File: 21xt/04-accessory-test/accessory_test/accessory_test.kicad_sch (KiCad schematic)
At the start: 10 parts, among them J1 Conn_01x44, J2 Conn_01x01, J3 Conn_01x02, U3 Teensy4.1

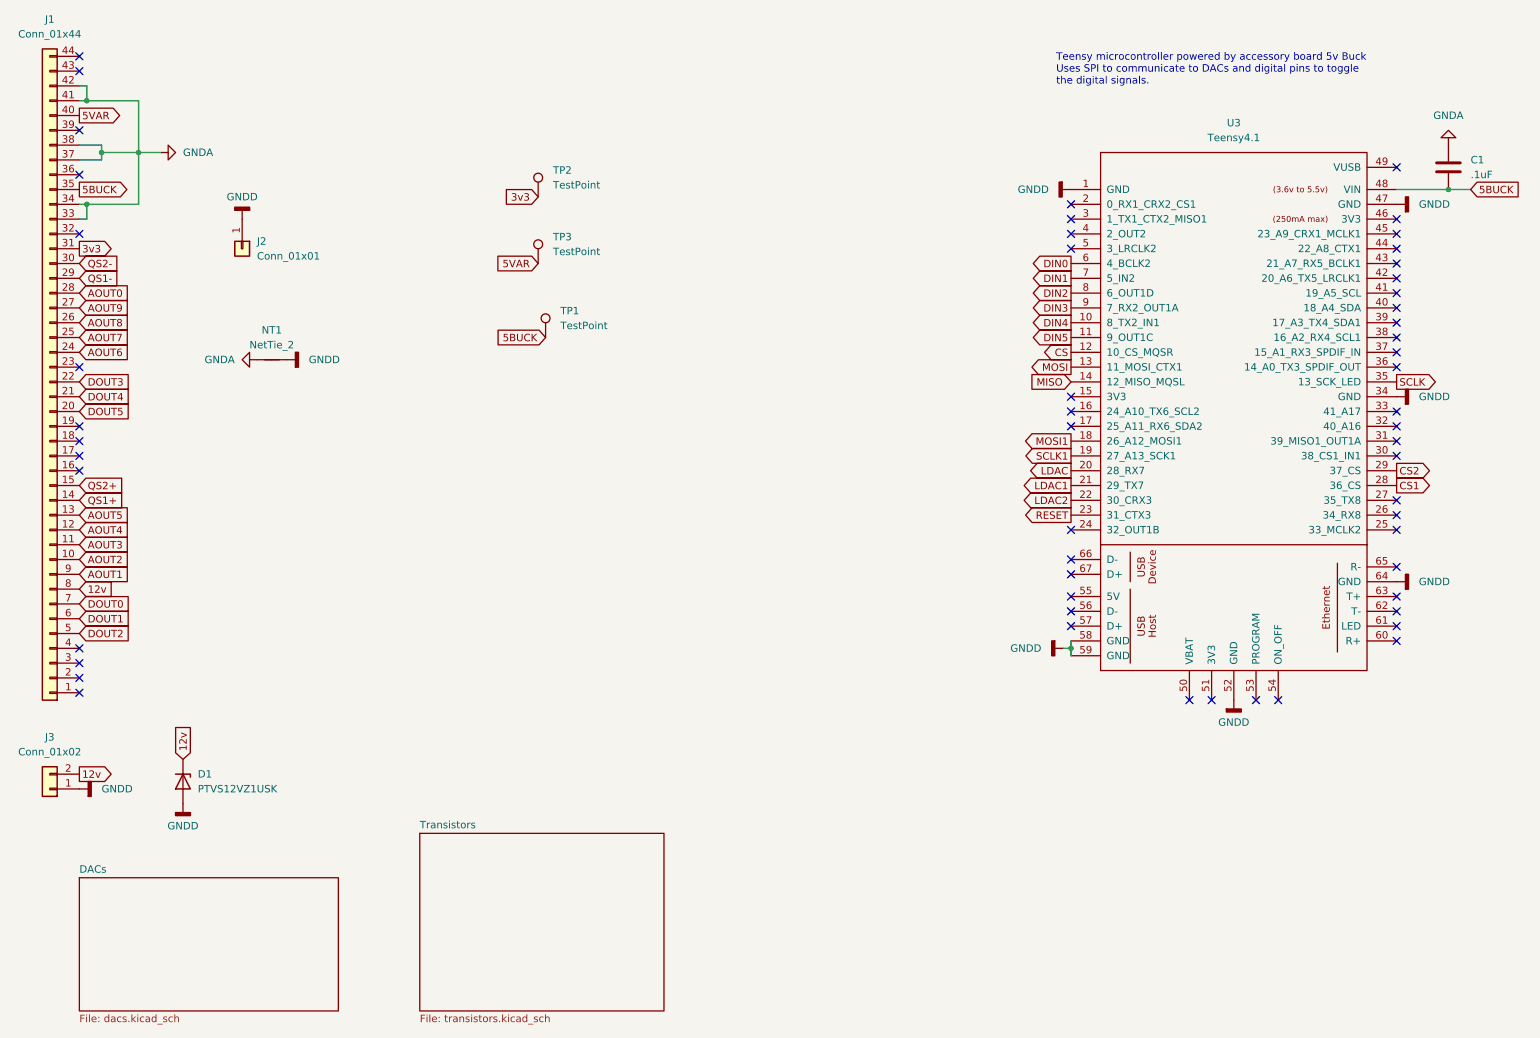
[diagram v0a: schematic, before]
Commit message: finish max5719 breakout board
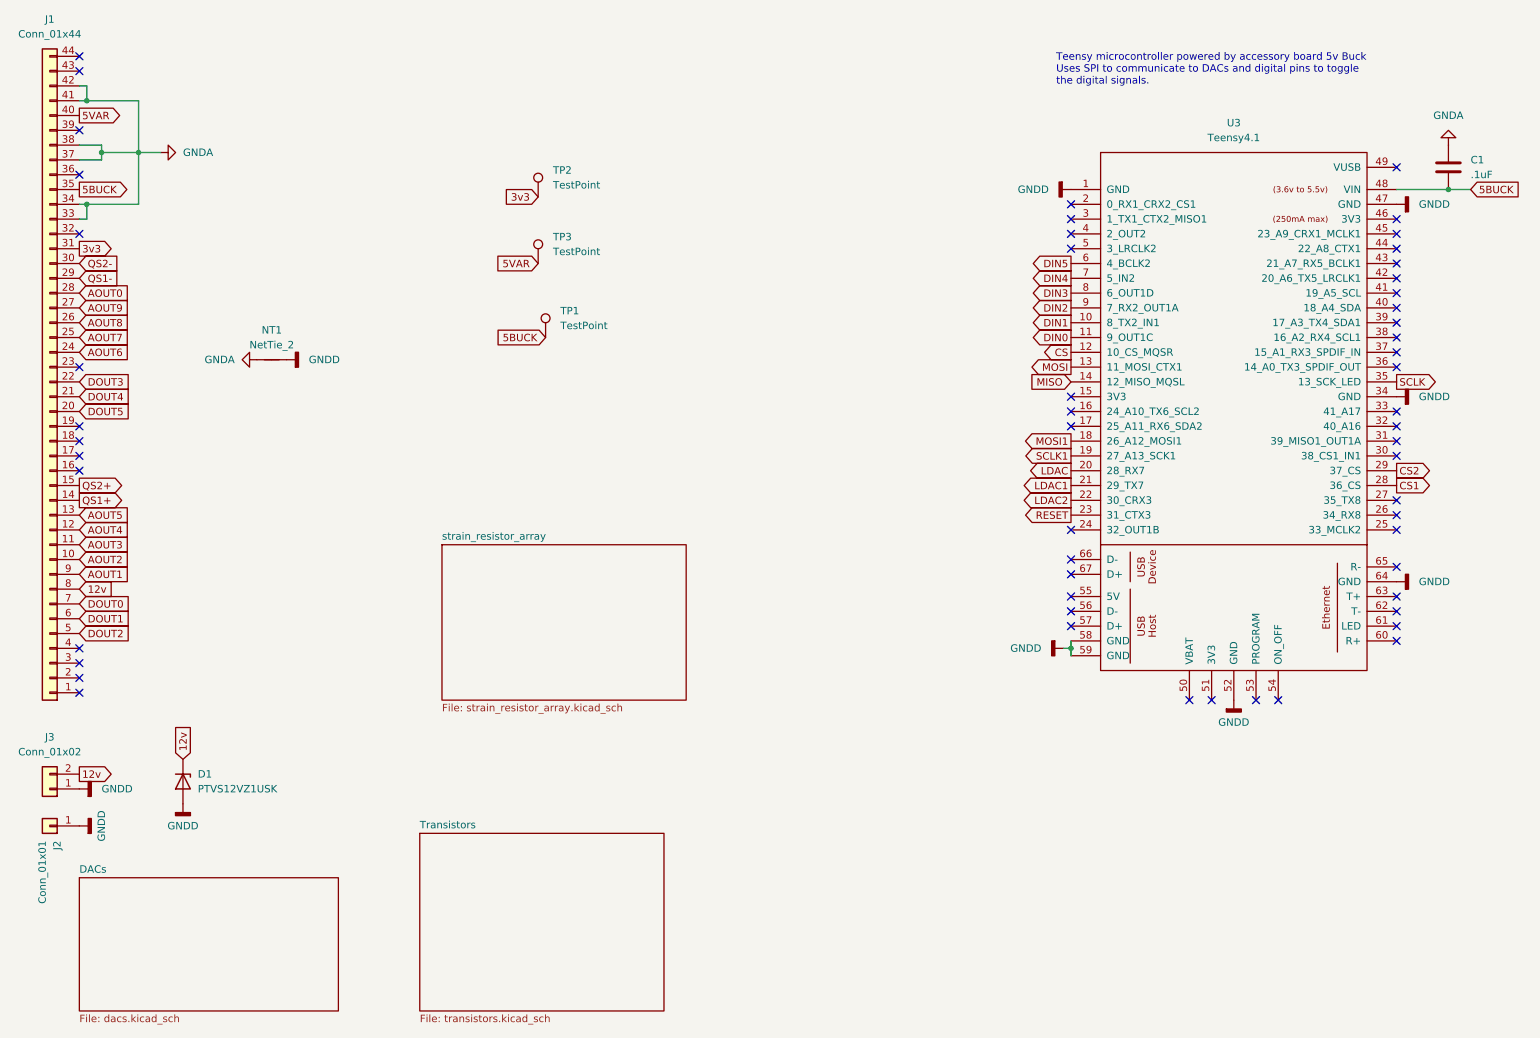
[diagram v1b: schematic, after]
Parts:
- U3: footprint accessory_test:teensy4.1 -> accessory_test:Teensy41
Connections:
- net DIN0: now also U3.11 (9_OUT1C); no longer U3.6 (4_BCLK2)
- net DIN1: now also U3.10 (8_TX2_IN1); no longer U3.7 (5_IN2)
- net DIN2: now also U3.9 (7_RX2_OUT1A); no longer U3.8 (6_OUT1D)
- net DIN3: now also U3.8 (6_OUT1D); no longer U3.9 (7_RX2_OUT1A)
- net DIN4: now also U3.7 (5_IN2); no longer U3.10 (8_TX2_IN1)
- net DIN5: now also U3.6 (4_BCLK2); no longer U3.11 (9_OUT1C)
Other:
- added sheet strain_resistor_array (strain_resistor_array.kicad_sch)
- moved on the sheet: J2

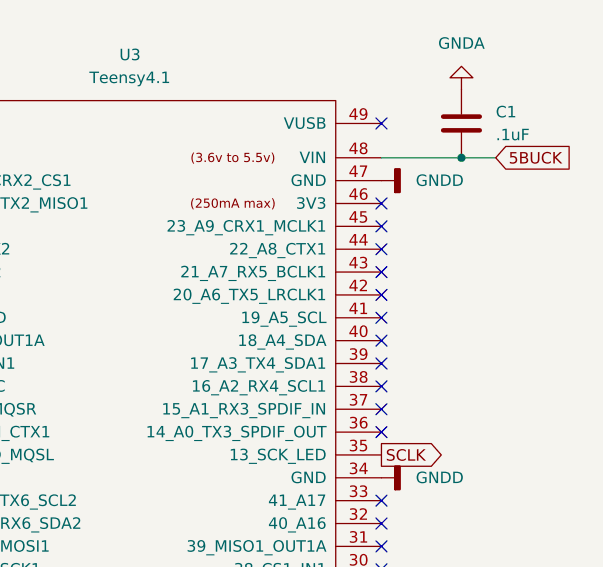
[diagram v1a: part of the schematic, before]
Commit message: finish max5719 breakout board
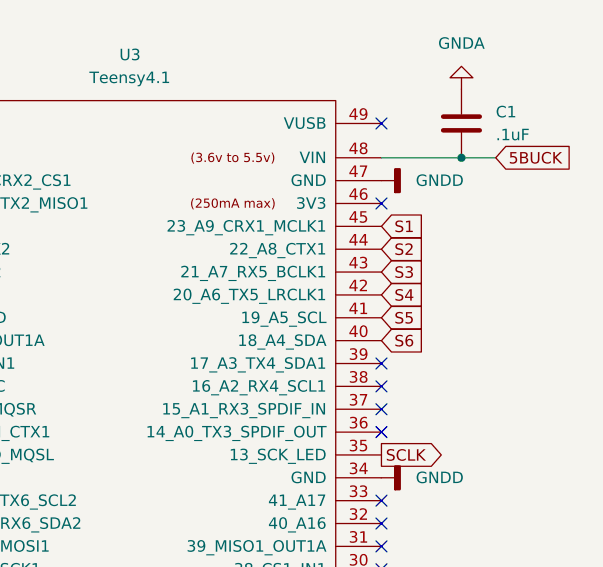
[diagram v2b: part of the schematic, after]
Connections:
- net S6: now reaches U3.40 (18_A4_SDA)
- net S5: now reaches U3.41 (19_A5_SCL)
- net S4: now reaches U3.42 (20_A6_TX5_LRCLK1)
- net S3: now reaches U3.43 (21_A7_RX5_BCLK1)
- net S2: now reaches U3.44 (22_A8_CTX1)
- net S1: now reaches U3.45 (23_A9_CRX1_MCLK1)
- no-connect marks 55 -> 49
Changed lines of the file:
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@@
-	)
-	(no_connect
-		(at 251.46 63.5)
-	)
-	(no_connect
-		(at 251.46 58.42)
 	)
 	(no_connect
@@
 	)
 	(no_connect
-		(at 251.46 66.04)
-	)
-	(no_connect
 		(at 25.4 91.44)
 	)
@@
 	)
 	(no_connect
-		(at 251.46 55.88)
-	)
-	(no_connect
 		(at 219.71 133.35)
 	)
@@
 	)
 	(no_connect
-		(at 251.46 60.96)
-	)
-	(no_connect
 		(at 251.46 88.9)
 	)
@@
 	(no_connect
 		(at 251.46 50.8)
-	)
-	(no_connect
-		(at 251.46 53.34)
 	)
 	(no_connect
@@
 		)
 	)
+	(global_label "S2"
+		(shape input)
+		(at 251.46 55.88 0)
+		(fields_autoplaced yes)
+		(effects
+			(font
+				(size 1.27 1.27)
+			)
+			(justify left)
+		)
+		(property "Intersheetrefs" "${INTERSHEET_REFS}"
+			(at 256.8642 55.88 0)
+			(effects
+				(font
+					(size 1.27 1.27)
+				)
+				(justify left)
+				(hide yes)
+			)
+		)
+	)
+	(global_label "S3"
+		(shape input)
+		(at 251.46 58.42 0)
+		(fields_autoplaced yes)
+		(effects
+			(font
+				(size 1.27 1.27)
+			)
+			(justify left)
+		)
+		(property "Intersheetrefs" "${INTERSHEET_REFS}"
+			(at 256.8642 58.42 0)
+			(effects
+				(font
+					(size 1.27 1.27)
+				)
+				(justify left)
+				(hide yes)
+			)
+		)
+	)
 	(global_label "DOUT1"
 		(shape input)
@@
 		)
 	)
+	(global_label "S4"
+		(shape input)
+		(at 251.46 60.96 0)
+		(fields_autoplaced yes)
+		(effects
+			(font
+				(size 1.27 1.27)
+			)
+			(justify left)
+		)
+		(property "Intersheetrefs" "${INTERSHEET_REFS}"
+			(at 256.8642 60.96 0)
+			(effects
+				(font
+					(size 1.27 1.27)
+				)
+				(justify left)
+				(hide yes)
+			)
+		)
+	)
 	(global_label "SCLK"
 		(shape output)
@@
 		)
 	)
+	(global_label "S1"
+		(shape input)
+		(at 251.46 53.34 0)
+		(fields_autoplaced yes)
+		(effects
+			(font
+				(size 1.27 1.27)
+			)
+			(justify left)
+		)
+		(property "Intersheetrefs" "${INTERSHEET_REFS}"
+			(at 256.8642 53.34 0)
+			(effects
+				(font
+					(size 1.27 1.27)
+				)
+				(justify left)
+				(hide yes)
+			)
+		)
+	)
 	(global_label "DOUT3"
 		(shape input)
@@
 		)
 	)
+	(global_label "S6"
+		(shape input)
+		(at 251.46 66.04 0)
+		(fields_autoplaced yes)
+		(effects
+			(font
+				(size 1.27 1.27)
+			)
+			(justify left)
+		)
+		(property "Intersheetrefs" "${INTERSHEET_REFS}"
+			(at 256.8642 66.04 0)
+			(effects
+				(font
+					(size 1.27 1.27)
+				)
+				(justify left)
+				(hide yes)
+			)
+		)
+	)
 	(global_label "DIN0"
 		(shape output)
@@
 			(effects
 				(font
+					(size 1.27 1.27)
+				)
+				(justify left)
+				(hide yes)
+			)
+		)
+	)
+	(global_label "S5"
+		(shape input)
+		(at 251.46 63.5 0)
+		(fields_autoplaced yes)
+		(effects
+			(font
+				(size 1.27 1.27)
+			)
+			(justify left)
+		)
+		(property "Intersheetrefs" "${INTERSHEET_REFS}"
+			(at 256.8642 63.5 0)
+			(effects
+				(font
